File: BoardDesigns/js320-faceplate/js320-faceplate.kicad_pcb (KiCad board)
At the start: 2 copper layers, 95 x 24.7 mm, 15 parts, among them J1 JS220, J2 Barrel_Jack, J3 Conn_01x04_Socket, SW1 SS-10-23NP-LE, U1 LT3045xDD, U2 XC6206PxxxMR

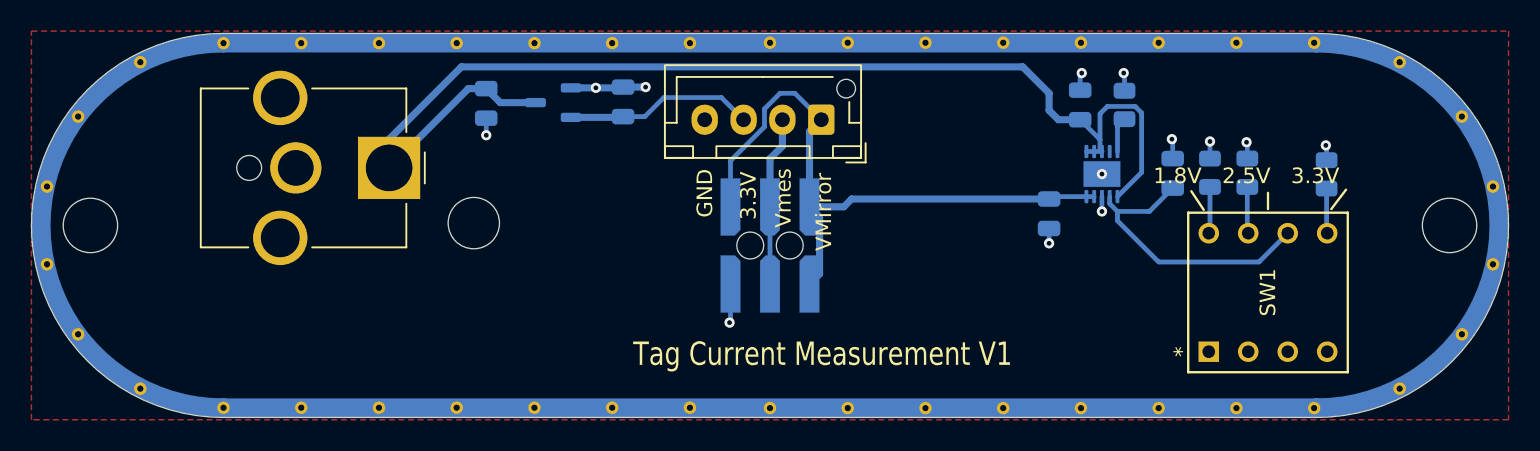
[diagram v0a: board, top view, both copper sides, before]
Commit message: checkpoint
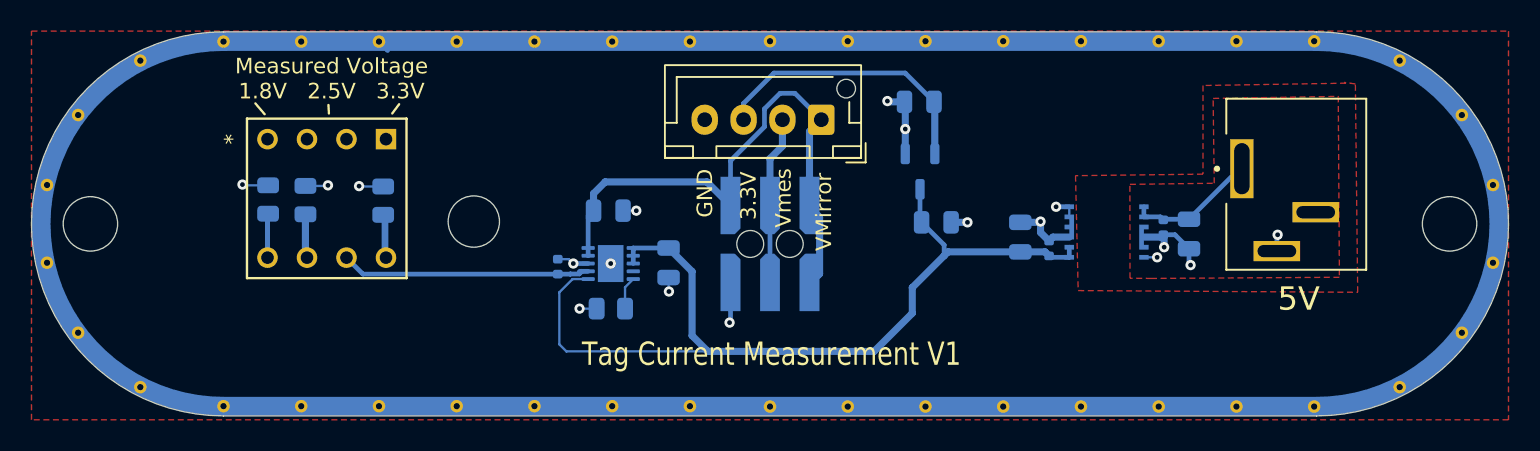
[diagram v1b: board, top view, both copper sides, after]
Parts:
- removed J2: Barrel_Jack, Connector_BarrelJack:BarrelJack_CUI_PJ-063AH_Horizontal_CircularHoles
- added C10: 22nf, Capacitor_SMD:C_0402_1005Metric, B.Cu at (156.4, 81.5)
- added C7: 22nf, Capacitor_SMD:C_0402_1005Metric, B.Cu at (163.8, 80.1)
- added C8: 22uf, Capacitor_SMD:C_0805_2012Metric, B.Cu at (154.6, 80.8)
- added C9: 10uf, Capacitor_SMD:C_0805_2012Metric, B.Cu at (165.4, 80.5)
- added J4: 54-00286, libraries:TENSILITY_54-00286, F.Cu at (172.3, 77.3)
- added U4: PUCC33420RAQR, libraries:VSON-FCRLF12_RAQ_TEX, B.Cu at (160.2, 80.4)
- C2: value 4.7uf -> 22nf; footprint Capacitor_SMD:C_0805_2012Metric -> Capacitor_SMD:C_0402_1005Metric
- C3: value 4.7uf -> 10uf
- R1: value 18K -> 18k
- R2: value 24.9K -> 24k
- R3: value 33K -> 33k
- R4: value 1K -> 1k
- SW1: value SS-10-23NP-LE -> SS-10-23NPE
- moved R1 60.7 mm to (113.6, 78.4)
- moved R2 60.6 mm to (108.6, 78.4)
- moved R3 60.6 mm to (106.2, 78.3)
- moved SW1 54.7 mm to (113.8, 74.5), turned to -90 degrees
- moved C2 40.0 mm to (124.8, 82.7)
- moved R4 35.5 mm to (128.3, 85.3), turned to 0 degrees
- moved U1 32.1 mm to (128.3, 82.5), turned to 180 degrees
- moved C4 29.9 mm to (149.2, 79.8), turned to 0 degrees
- moved C1 28.4 mm to (132.0, 82.4), turned to -90 degrees
- moved C3 28.4 mm to (128.1, 79.0), turned to 0 degrees
- moved U2 24.0 mm to (148.2, 76.5), turned to -90 degrees
- moved C5 19.0 mm to (148.1, 72.0), turned to 180 degrees
- moved J1 0.10 mm to (138.5, 79.9)
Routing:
- net /vin: track 76.5 -> 58.9 mm
- net /VINP: track 0.00 -> 8.39 mm
- net GNDPWR: track 0.00 -> 7.17 mm, vias 0 -> 4
- net GND: track 17.2 -> 23.7 mm, vias 13 -> 14
- net +3.3V: track 12.2 -> 18.2 mm
- net /Vprog: track 42.0 -> 37.6 mm
- net Net-(R1-Pad1): track 2.89 -> 5.72 mm
- net Net-(R3-Pad1): track 3.01 -> 5.68 mm
- net /sens: track 18.7 -> 16.3 mm
- added copper zone on F.Cu, net GNDPWR
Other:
- board text added: "5V"
- board text added: "Measured Voltage 1.8V 2.5V 3.3V"
- board text removed: "1.8V 2.5V 3.3V"
